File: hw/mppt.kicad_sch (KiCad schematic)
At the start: 4 parts

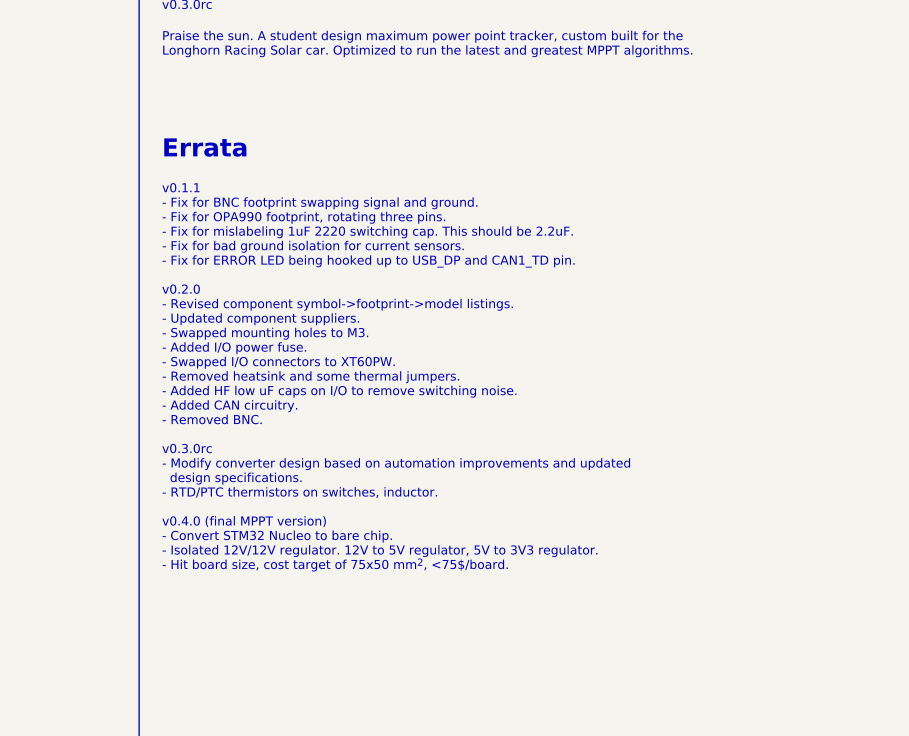
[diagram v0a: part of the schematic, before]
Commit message: savestate
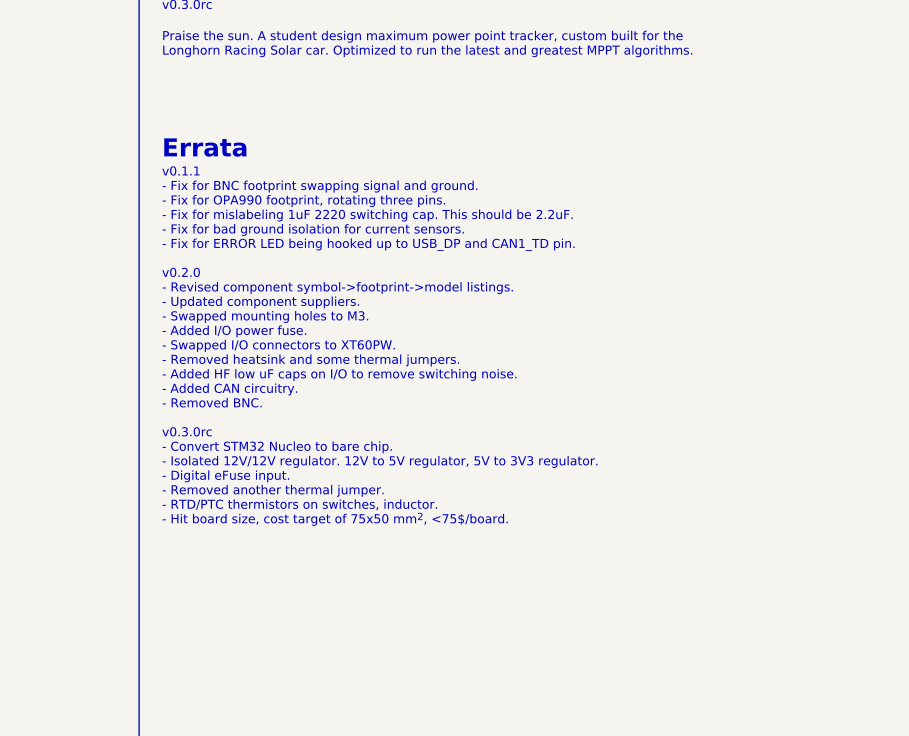
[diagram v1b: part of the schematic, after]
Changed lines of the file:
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@@
     (effects (font (size 2 2) (thickness 0.4) bold) (justify left bottom))
   )
-  (text "v0.1.1\n- Fix for BNC footprint swapping signal and ground.\n- Fix for OPA990 footprint, rotating three pins.\n- Fix for mislabeling 1uF 2220 switching cap. This should be 2.2uF.\n- Fix for bad ground isolation for current sensors.\n- Fix for ERROR LED being hooked up to USB_DP and CAN1_TD pin.\n\nv0.2.0\n- Revised component symbol->footprint->model listings.\n- Updated component suppliers.\n- Swapped mounting holes to M3.\n- Added I/O power fuse.\n- Swapped I/O connectors to XT60PW.\n- Removed heatsink and some thermal jumpers.\n- Added HF low uF caps on I/O to remove switching noise.\n- Added CAN circuitry.\n- Removed BNC.\n\nv0.3.0rc\n- Modify converter design based on automation improvements and updated\n  design specifications.\n- RTD/PTC thermistors on switches, inductor.\n\nv0.4.0 (final MPPT version)\n- Convert STM32 Nucleo to bare chip.\n- Isolated 12V/12V regulator. 12V to 5V regulator, 5V to 3V3 regulator.\n- Hit board size, cost target of 75x50 mm^{2}, <75$/board.\n"
-    (at 176.53 90.17 0)
+  (text "v0.1.1\n- Fix for BNC footprint swapping signal and ground.\n- Fix for OPA990 footprint, rotating three pins.\n- Fix for mislabeling 1uF 2220 switching cap. This should be 2.2uF.\n- Fix for bad ground isolation for current sensors.\n- Fix for ERROR LED being hooked up to USB_DP and CAN1_TD pin.\n\nv0.2.0\n- Revised component symbol->footprint->model listings.\n- Updated component suppliers.\n- Swapped mounting holes to M3.\n- Added I/O power fuse.\n- Swapped I/O connectors to XT60PW.\n- Removed heatsink and some thermal jumpers.\n- Added HF low uF caps on I/O to remove switching noise.\n- Added CAN circuitry.\n- Removed BNC.\n\nv0.3.0rc\n- Convert STM32 Nucleo to bare chip.\n- Isolated 12V/12V regulator. 12V to 5V regulator, 5V to 3V3 regulator.\n- Digital eFuse input.\n- Removed another thermal jumper.\n- RTD/PTC thermistors on switches, inductor.\n- Hit board size, cost target of 75x50 mm^{2}, <75$/board.\n"
+    (at 176.53 85.09 0)
     (effects (font (size 1 1)) (justify left bottom))
   )
